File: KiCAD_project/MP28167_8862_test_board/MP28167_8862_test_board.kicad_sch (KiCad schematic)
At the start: 34 parts, among them IC1 MP8862GQ-0000-Z, J1 Conn_01x04_Male, J2 Conn_01x02_Female, J3 Conn_01x02_Female, J4 Conn_01x02_Female, J5 Conn_01x02_Female, U1 AP63203WU

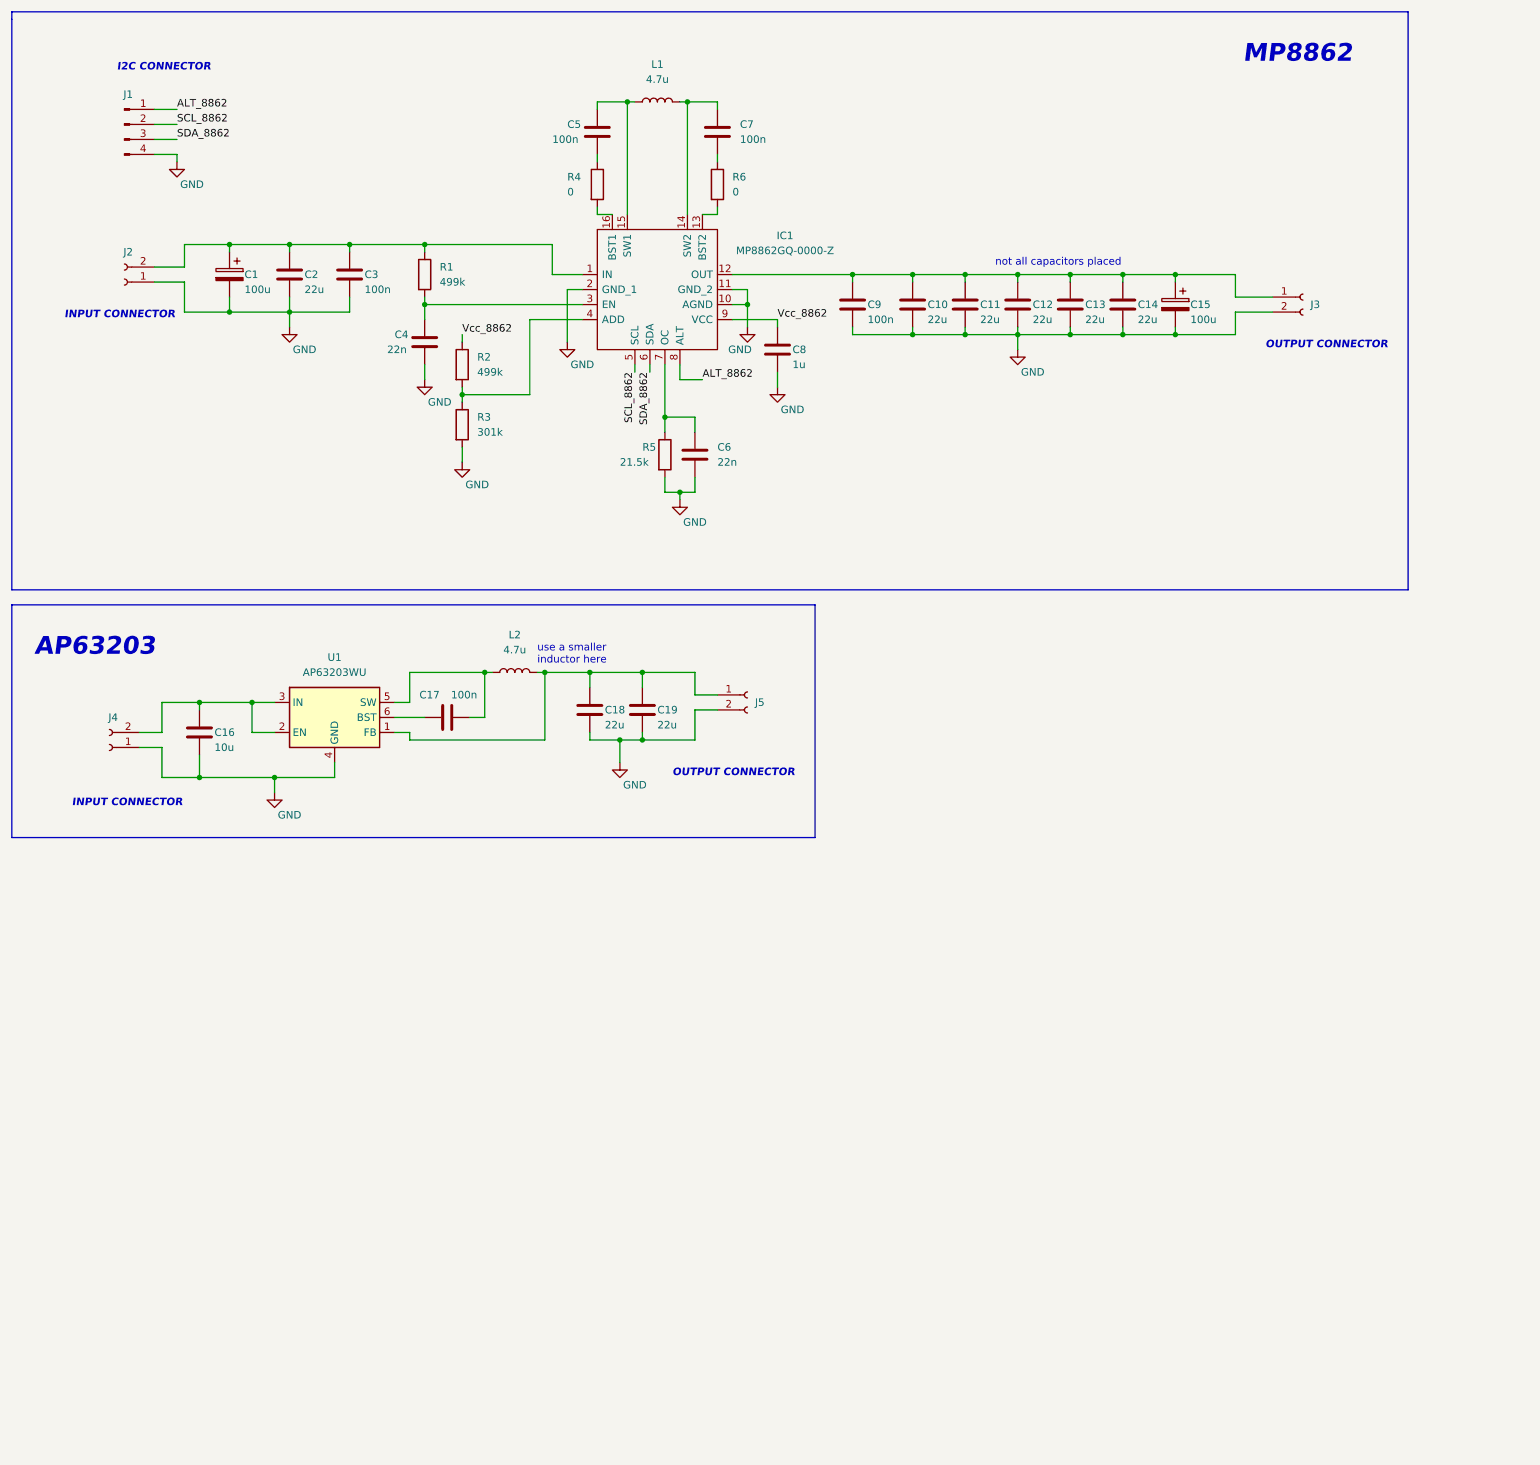
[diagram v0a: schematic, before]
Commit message: first schematic
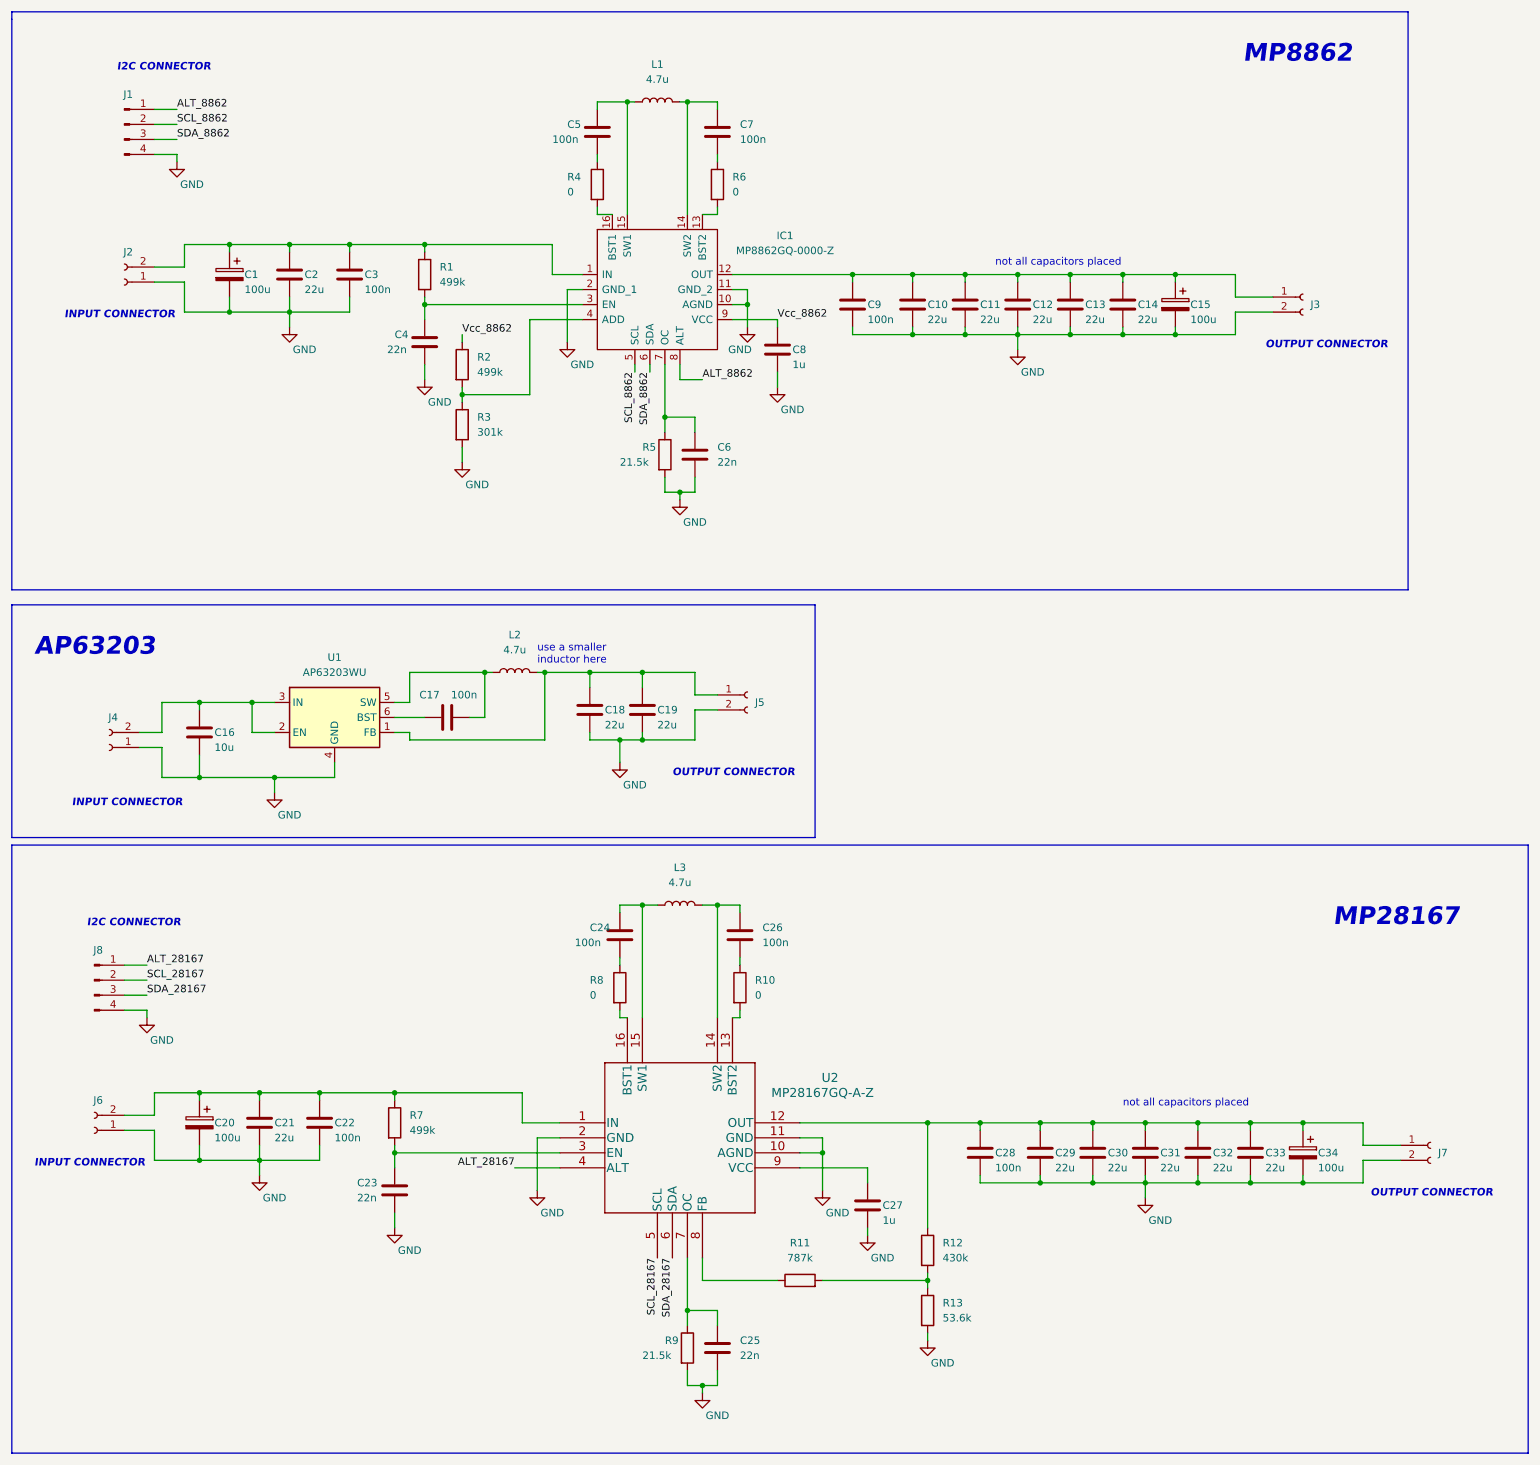
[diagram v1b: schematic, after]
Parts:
- added C20, C34: 100u, symbol Device:C_Polarized
- added C21, C29, C30, C31, C32, C33: 22u, symbol Device:C
- added C22, C24, C26, C28: 100n, symbol Device:C
- added C23, C25: 22n, symbol Device:C
- added C27: 1u, symbol Device:C
- added J6, J7: Conn_01x02_Female, symbol Connector:Conn_01x02_Female
- added J8: Conn_01x04_Male, symbol Connector:Conn_01x04_Male
- added L3: 4.7u, symbol Device:L
- added R10, R8: 0, symbol Device:R
- added R11: 787k, symbol Device:R
- added R12: 430k, symbol Device:R
- added R13: 53.6k, symbol Device:R
- added R7: 499k, symbol Device:R
- added R9: 21.5k, symbol Device:R
- added U2: MP28167GQ-A-Z, QFN-16_MP28167_MNP, symbol 2023-03-10_09-43-26:MP28167GQ-A-Z
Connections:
- net GND: now also C20.2, C21.2, C22.2, C23.2, C25.2, C27.2, C28.2, C29.2, C30.2, C31.2, C32.2, C33.2, C34.2, J6.1 (Pin_1), J7.2 (Pin_2), J8.4 (Pin_4), R13.2, R9.2, U2.10 (AGND), U2.11 (GND), U2.2 (GND)
- new net: C24.2, R8.1
- new net: R8.2, U2.16 (BST1)
- new net: C20.1, C21.1, C22.1, J6.2 (Pin_2), R7.1, U2.1 (IN)
- new net: C28.1, C29.1, C30.1, C31.1, C32.1, C33.1, C34.1, J7.1 (Pin_1), R12.1, U2.12 (OUT)
- new net: C26.2, R10.1
- new net: R10.2, U2.13 (BST2)
- new net: C23.1, R7.2, U2.3 (EN)
- new net: C26.1, L3.2, U2.14 (SW2)
- new net: C24.1, L3.1, U2.15 (SW1)
- new net: C25.1, R9.1, U2.7 (OC)
- new net: R11.1, U2.8 (FB)
- new net: C27.1, U2.9 (VCC)
- new net: R11.2, R12.2, R13.1
- new net ALT_28167: J8.1 (Pin_1), U2.4 (ALT)
- new net SCL_28167: J8.2 (Pin_2), U2.5 (SCL)
- new net SDA_28167: J8.3 (Pin_3), U2.6 (SDA)
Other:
- note added: "MP28167"
- title: (none) -> PM8862 / PM28167 dev board

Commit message: footprint update
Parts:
- U2: footprint QFN-16_MP28167_MNP -> footprints:MP28167GQ-A-Z
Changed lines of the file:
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@@
       (effects (font (size 1.524 1.524)))
     )
-    (property "Footprint" "QFN-16_MP28167_MNP" (id 2) (at 127 190.754 0)
+    (property "Footprint" "footprints:MP28167GQ-A-Z" (id 2) (at 127 190.754 0)
       (effects (font (size 1.524 1.524)) hide)
     )
@@
     )
     (path "/82d40548-c1ae-451b-bea2-e6eb9c8d37b8"
-      (reference "U2") (unit 1) (value "MP28167GQ-A-Z") (footprint "QFN-16_MP28167_MNP")
-    )
-  )
+      (reference "U2") (unit 1) (value "MP28167GQ-A-Z") (footprint "footprints:MP28167GQ-A-Z")
+    )
+  )

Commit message: pcb layout update
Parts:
- C1, C15, C20, C34: footprint (none) -> Capacitor_SMD:CP_Elec_5x5.3
- C10, C11, C12, C13, C14, C16, C17, C18, C19, C21, C24, C26, C29, C3, C30, C31, C32, C33, C5, C7, C9: footprint (none) -> Capacitor_SMD:C_0805_2012Metric_Pad1.18x1.45mm_HandSolder
- C2, C22, C23, C25, C27, C28, C4, C6, C8: footprint (none) -> Capacitor_SMD:C_0603_1608Metric_Pad1.08x0.95mm_HandSolder
- J1, J8: footprint (none) -> Connector_PinHeader_2.54mm:PinHeader_1x04_P2.54mm_Vertical
- J2, J3, J4, J5, J6, J7: footprint (none) -> Connector_Wire:SolderWire-0.1sqmm_1x02_P3.6mm_D0.4mm_OD1mm
- L1, L3: footprint (none) -> footprints:EXL1V0705 inductor
- L2: footprint (none) -> footprints:SDES064T-4R7MS inductor
- R1, R10, R11, R12, R13, R2, R3, R4, R5, R6, R7, R8, R9: footprint (none) -> Resistor_SMD:R_0603_1608Metric_Pad0.98x0.95mm_HandSolder
